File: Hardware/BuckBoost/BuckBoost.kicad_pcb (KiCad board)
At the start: 2 copper layers, 18.5 x 13 mm, 12 parts, among them J1 Screw_Terminal_01x04, U1 ISL85415FRZ

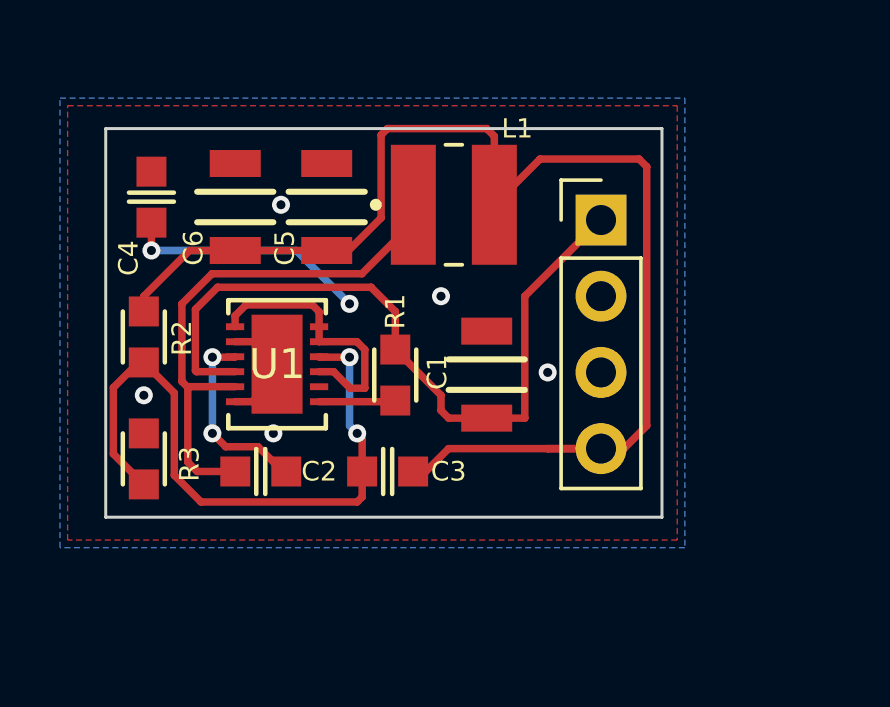
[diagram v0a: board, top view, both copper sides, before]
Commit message: feat: Update PCB
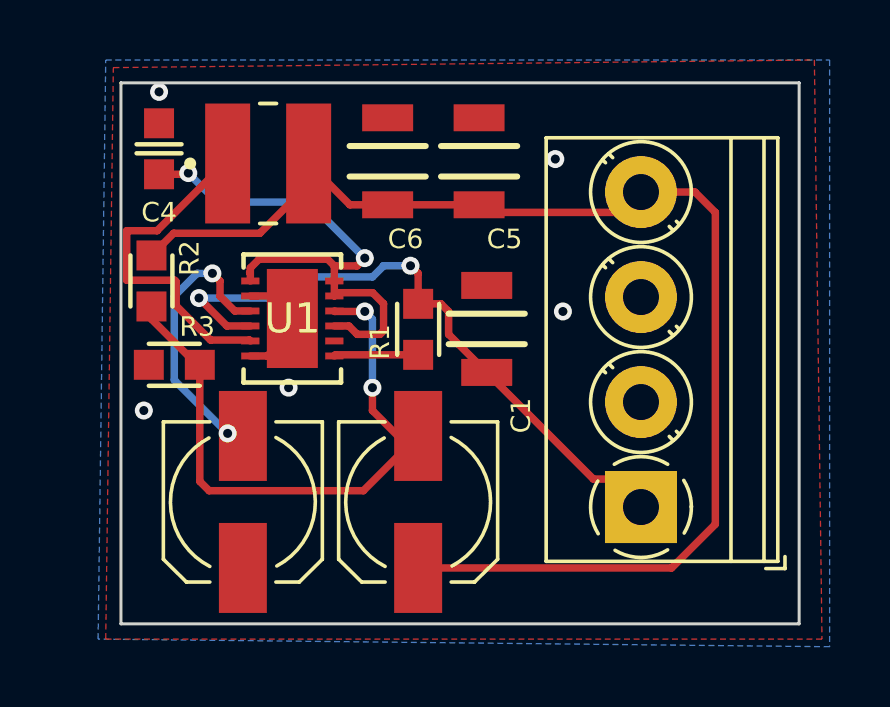
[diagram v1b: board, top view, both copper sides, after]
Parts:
- C2, C3: footprint PCM_4ms_Capacitor:C_0603 -> PCM_4ms_Capacitor:CP_Elec_5x5.3
- J1: footprint Connector_PinHeader_2.54mm:PinHeader_1x04_P2.54mm_Vertical -> TerminalBlock_Phoenix:TerminalBlock_Phoenix_PT-1,5-4-3.5-H_1x04_P3.50mm_Horizontal
- moved J1 9.66 mm to (153.0, 85.3), turned to 90 degrees
- moved L1 6.34 mm to (140.5, 73.8)
- moved C5 5.30 mm to (147.6, 73.7)
- moved C6 5.30 mm to (144.5, 73.7)
- moved R3 3.30 mm to (137.4, 80.5), turned to 180 degrees
- moved R2 1.88 mm to (136.7, 77.7)
- moved R1 1.70 mm to (145.5, 79.3)
- moved C4 1.63 mm to (136.9, 73.3)
- moved U1 1.61 mm to (141.3, 79.0)
- moved C1 1.52 mm to (147.8, 79.3)
- moved C3 1.44 mm to (145.5, 85.1), turned to 90 degrees
- moved C2 1.18 mm to (139.7, 85.1), turned to 90 degrees
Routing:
- net Net-(U1-PHASE): track 18.1 -> 11.8 mm
- net /VIN: track 25.2 -> 21.7 mm, vias 0 -> 2
- net Net-(U1-BOOT): track 6.29 -> 8.98 mm
- net /VOUT: track 41.6 -> 42.5 mm
- net Net-(U1-COMP): track 17.3 -> 18.2 mm
- net Net-(U1-FB): track 21.7 -> 21.0 mm
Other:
- board size 18.5 x 13 mm -> 22.6 x 18 mm
